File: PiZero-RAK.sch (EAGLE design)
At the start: 28 parts, among them J11 CON_HEADER_1X06-PTH, J2 CONN_20X2HLE, X1 SPTAF_23.5, X2 SPTAF_25.0MM

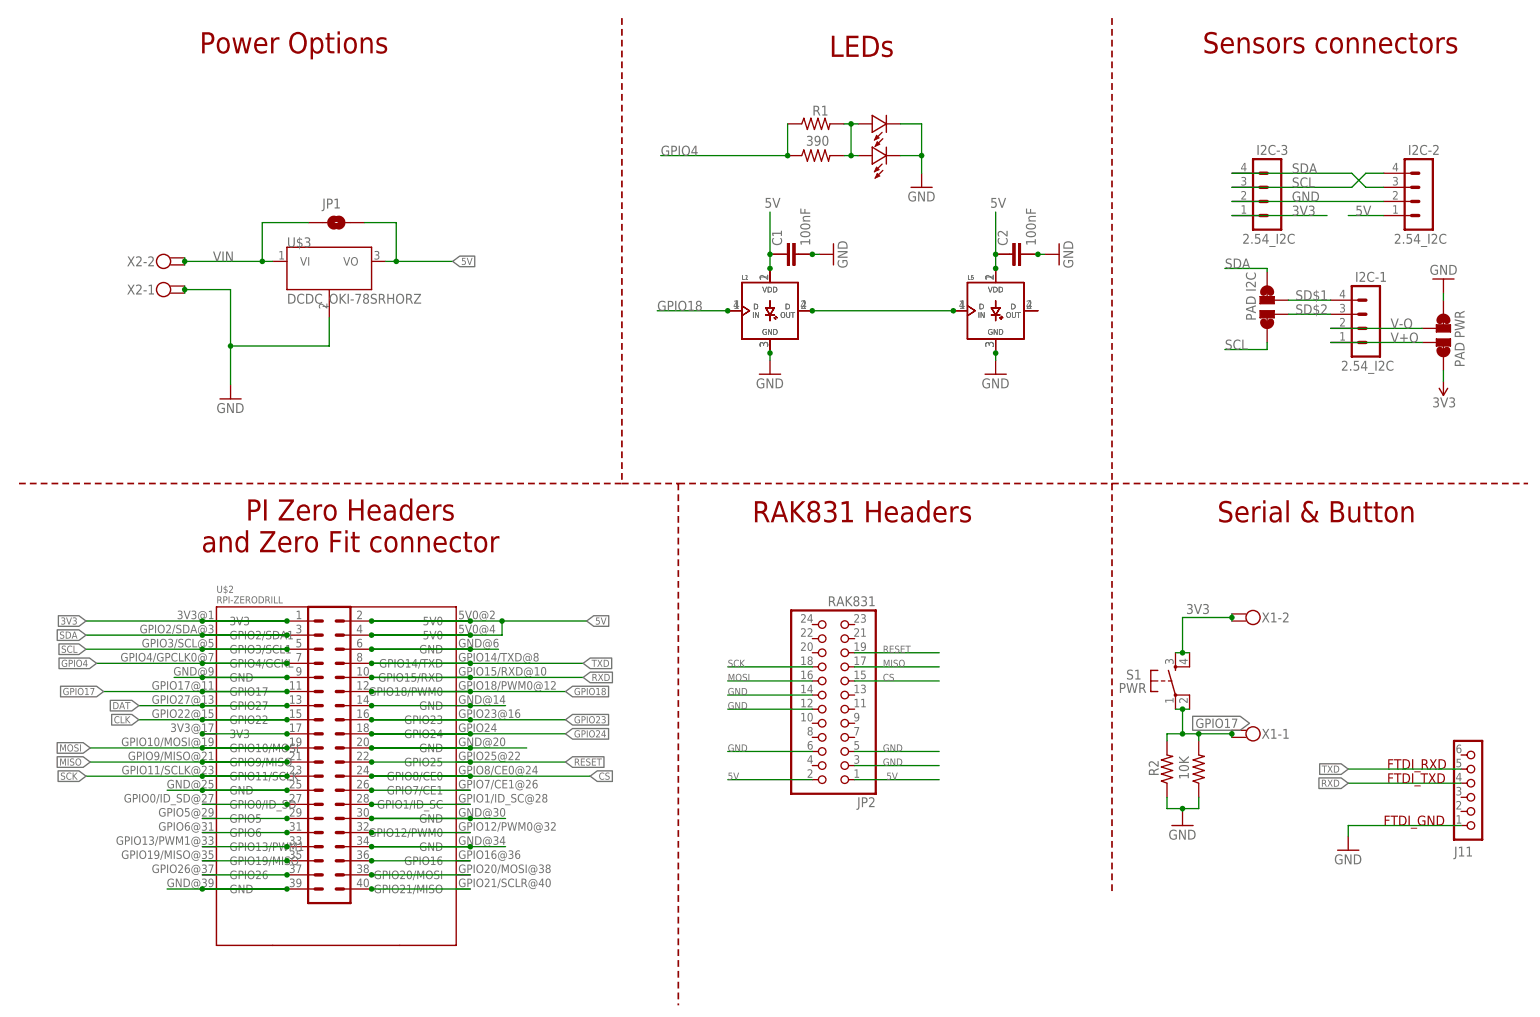
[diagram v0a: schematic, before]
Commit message: Bump to V1.5
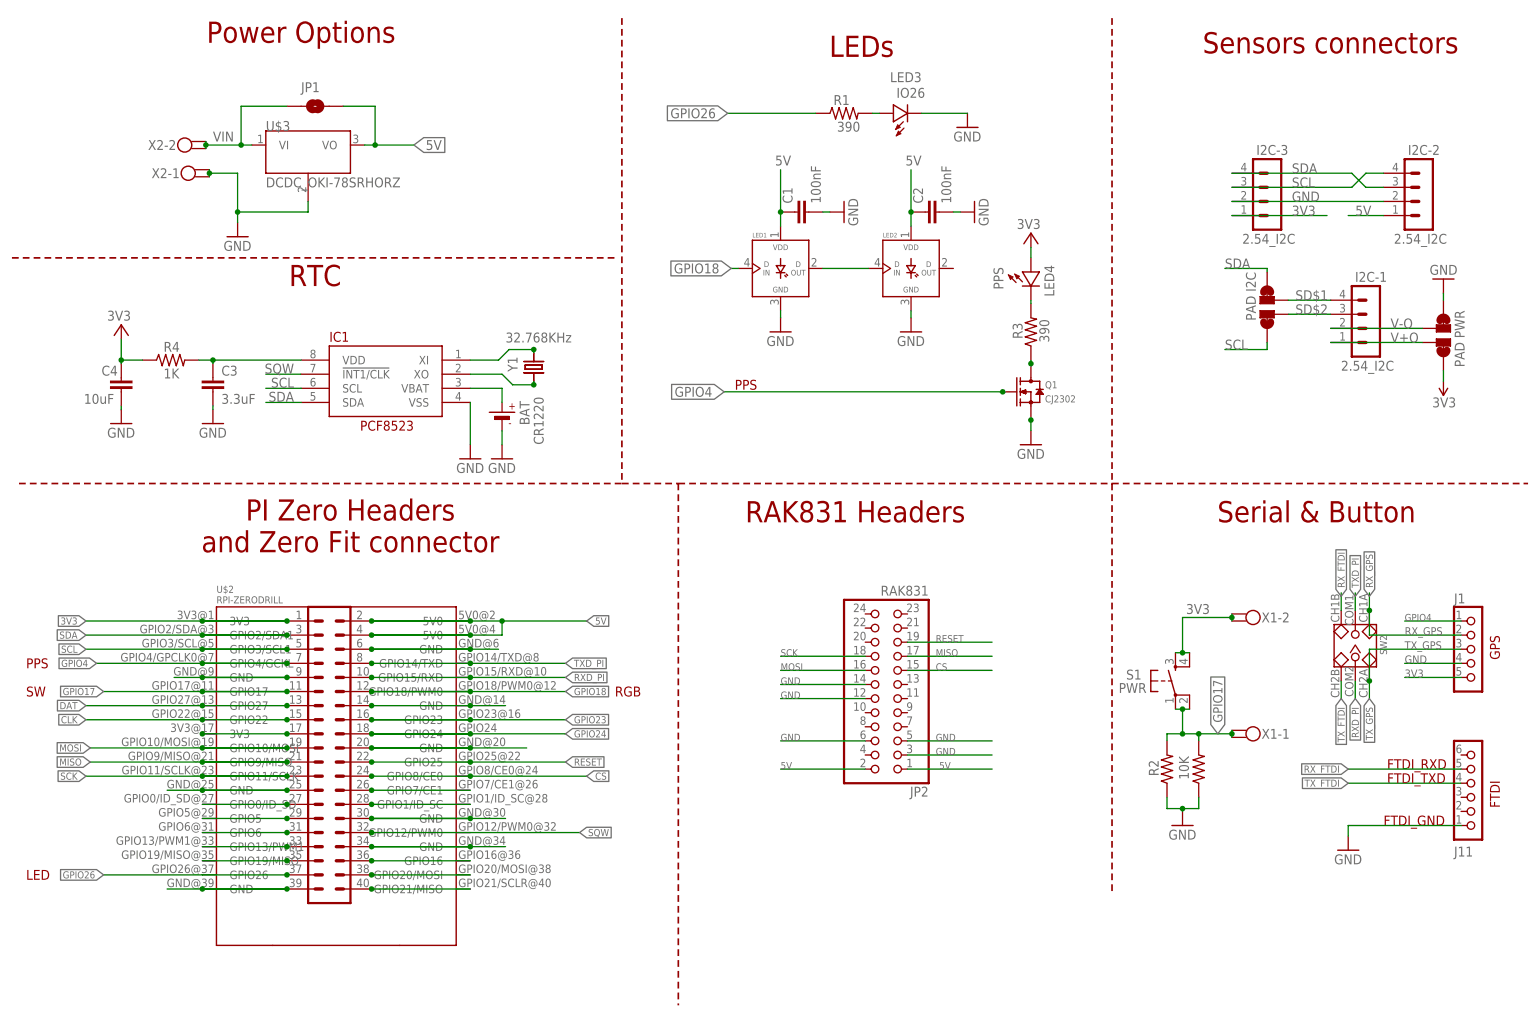
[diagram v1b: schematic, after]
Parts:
- removed C6: (no value), _c2h:CAPPTH
- removed L1, L5: WS2812BLONG, _c2h:WS2812BLONG
- removed L2, L6: WS2812BNOR, _c2h:WS2812BNOR
- removed R6: (no value), _c2h:RESISTOR0805-RES
- removed U$6: IO4, _c2h:LED3MM
- added BAT: CR1220, microbuilder:BATTERYCR1220_SMT
- added C3: 3.3uF, _c2h:CAP0805-CAP-LARGEPADS
- added IC1: PCF8523, microbuilder:RTC_PCF8523T
- added J1: CON_HEADER_1X05-PTH, dp_devices:CON_HEADER_1X05-PTH
- added LED1, LED2: WS2812BLONG, _c2h:WS2812BLONG
- added LED4: PPS, _c2h:LED0805-LARGE
- added Q1: CJ2302, Seeed-Transistor:SMD-MOSFET-N-CH-20V-2.1A-CJ2302(SOT-23)
- added R3: 390, _c2h:RESISTOR0805-RES
- added R4: 1K, _c2h:RESISTOR0805-RES
- added SW2: (no value), Seeed-Switch:DIP-TOGGLE-SWITCH-2CH-(2X3P-2.54)
- added Y1: 32.768KHz, adafruit:CRYSTALTC26H
- added Y2: (no value), microbuilder:CRYSTAL8X3.8SMT
- C4: value (none) -> 10uF; device _c2h:CAPPTH -> _c2h:CAP0805-CAP-LARGEPADS
- LED3: value LED0805 -> IO26; device _c2h:LED0805 -> _c2h:LED0805-LARGE
- R1: device _c2h:RESISTORPTH-1/4W -> _c2h:RESISTOR0805-RES
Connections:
- removed net N$18: L5.DOUT, L6.DOUT
- removed net N$29: J2.32, U$2.GPIO12/PWM0
- removed net RXD: J11.4, J2.10, U$2.GPIO15/RXD
- removed net TXD: J11.5, J2.8, U$2.GPIO14/TXD
- new net GPIO26: J2.37, R1.1, U$2.GPIO26
- new net N$26: IC1.XI, Y1.1, Y2.2
- new net N$27: Q1.D, R3.1
- new net N$38: IC1.XO, Y1.2, Y2.1
- new net RXD_PI: J2.10, SW2.COM2, U$2.GPIO15/RXD
- new net RX_FTDI: J11.5, SW2.CH1B
- new net RX_GPS: J1.2, SW2.CH1A
- new net SQW: IC1.!INT1/CLK, J2.32, U$2.GPIO12/PWM0
- new net TXD_PI: J2.8, SW2.COM1, U$2.GPIO14/TXD
- new net TX_FTDI: J11.4, SW2.CH2B
- new net TX_GPS: J1.3, SW2.CH2A
- new net VBAT: BAT.+, IC1.VBAT
- new net VDD: C3.1, IC1.VDD, R4.2
- net 3V3: now also C4.1, J1.5, LED4.PLUS, R4.1
- net 5V: now also LED1.VDD, LED2.VDD; no longer C4.1, C6.1, L1.VDD, L2.VDD, L5.VDD, L6.VDD
- net GND: now also BAT.-, C3.2, IC1.VSS, J1.4, LED1.GND, LED2.GND, Q1.S; no longer C6.2, L1.GND, L2.GND, L5.GND, L6.GND, U$6.MINUS
- net GPIO18: now also LED1.DIN; no longer L1.DIN, L2.DIN
- net GPIO4: now also J1.1, Q1.G; no longer R1.1, R6.1
- net N$16: no longer R6.2, U$6.PLUS
- net N$37: now also LED4.MINUS, R3.2; no longer J2.37, U$2.GPIO26
- net N$39: now also LED1.DOUT, LED2.DIN; no longer L1.DOUT, L2.DOUT, L5.DIN, L6.DIN
- net SCL: now also IC1.SCL
- net SDA: now also IC1.SDA
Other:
- note added: "FTDI"
- note added: "GPS"
- note added: "LED"
- note added: "PPS"
- note added: "RGB"
- note added: "RTC"
- note added: "SW"
- moved on the sheet: C1, C2, JP1, JP2, R1, U$3, X2-1, X2-2
